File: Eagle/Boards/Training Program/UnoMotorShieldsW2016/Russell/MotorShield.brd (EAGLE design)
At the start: 58.9 x 66 mm, 21 parts, among them J1 ARDUINO_UNO_R3

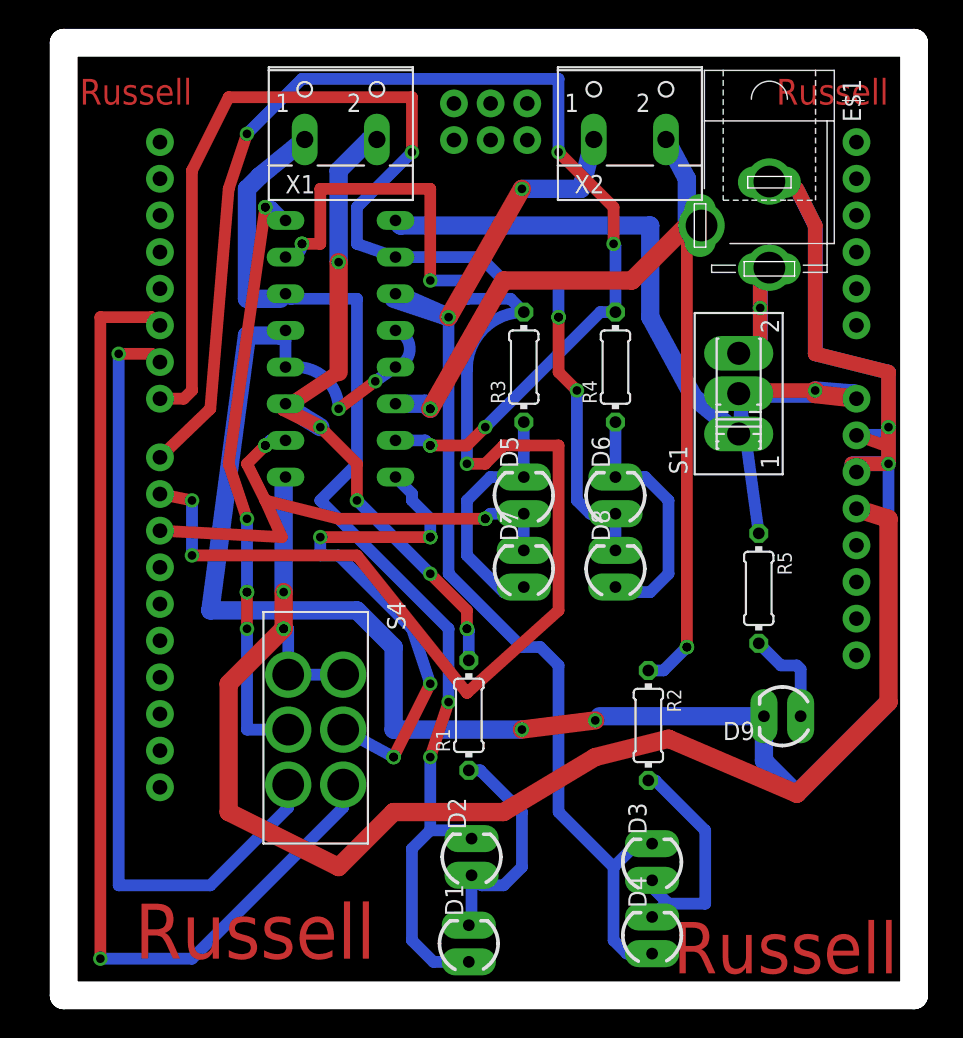
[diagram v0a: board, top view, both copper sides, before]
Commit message: compiled 1st board for fabrication
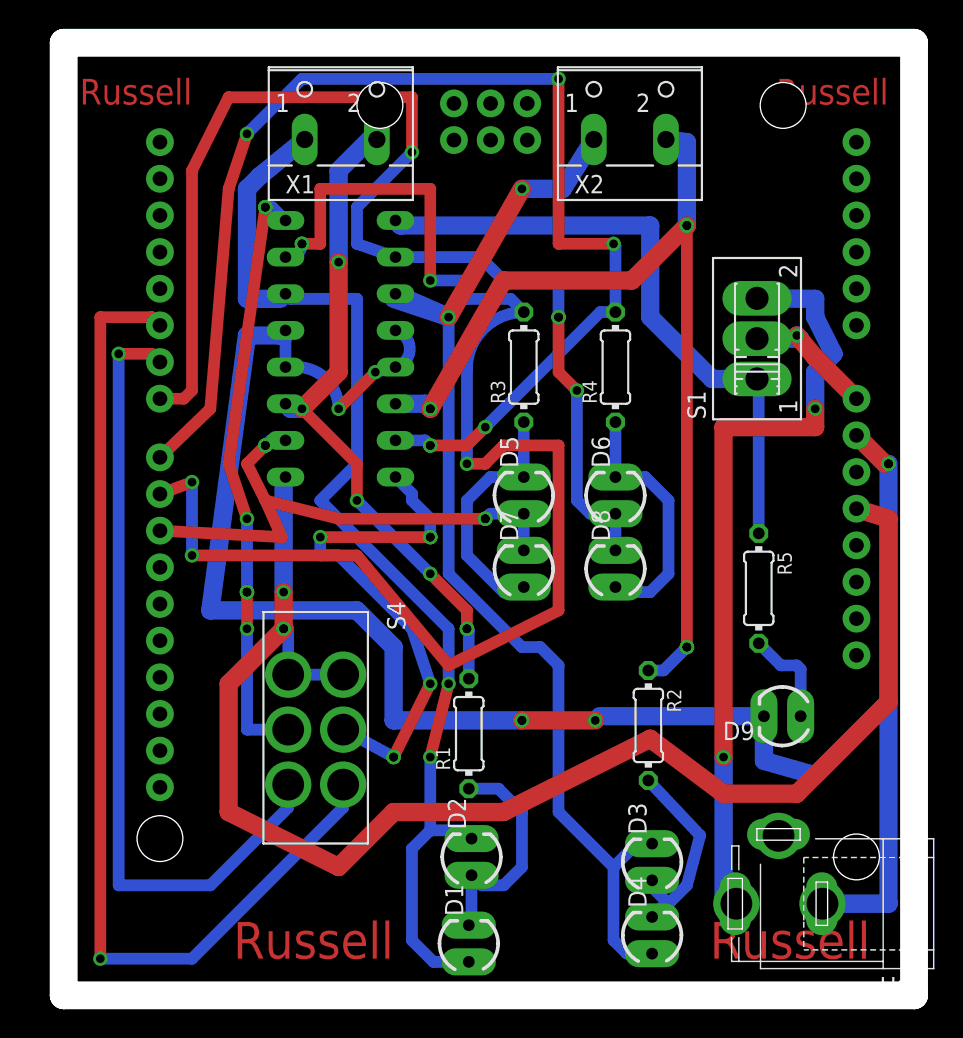
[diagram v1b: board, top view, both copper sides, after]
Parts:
- removed E$1: (no value), ISCTRainingProgram:5.5-2.5-BARRELCONNECTOR
- added U$2: BARREL_CONNECTOR, ISCTRainingProgram:5.5-2.5-BARRELCONNECTOR
- moved S1 4.02 mm to (49.3, 45.5)
- moved R1 1.27 mm to (29.3, 18.1)
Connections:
- removed net S$1: X2.2
- new net N$26: S1.3, U$2.3
- net N$1: now also X2.2
- net N$23: now also U$2.1
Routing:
- net N$26: track 0.00 -> 53.9 mm, vias 0 -> 2
- net N$2: track 53.6 -> 0.00 mm
- net N$23: track 119.7 -> 133.5 mm
- net S$2: track 10.2 -> 0.00 mm, vias 1 -> 0
- net N$4: track 19.0 -> 9.32 mm
- net N$1: track 59.6 -> 66.9 mm, vias 2 -> 3
- net S$1: track 6.32 -> 0.00 mm
- net N$3: track 48.3 -> 45.9 mm
- net N$18: track 16.6 -> 14.2 mm
- net N$6: track 46.3 -> 44.1 mm
- net N$11: track 84.3 -> 86.6 mm
- net N$12: track 97.4 -> 96.5 mm
- net N$10: track 82.5 -> 81.7 mm
- net N$21: track 16.5 -> 16.0 mm
